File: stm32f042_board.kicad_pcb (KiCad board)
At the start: 4 copper layers, 37.8 x 18.8 mm, 25 parts, among them J1 Conn_01x12_Female, J2 Conn_01x12_Female, J3 USB_B_Micro, J5 JTAG/SWD, U1 STM32F042F6Px, U2 MCP1802, U3 USBLC6-2SC6

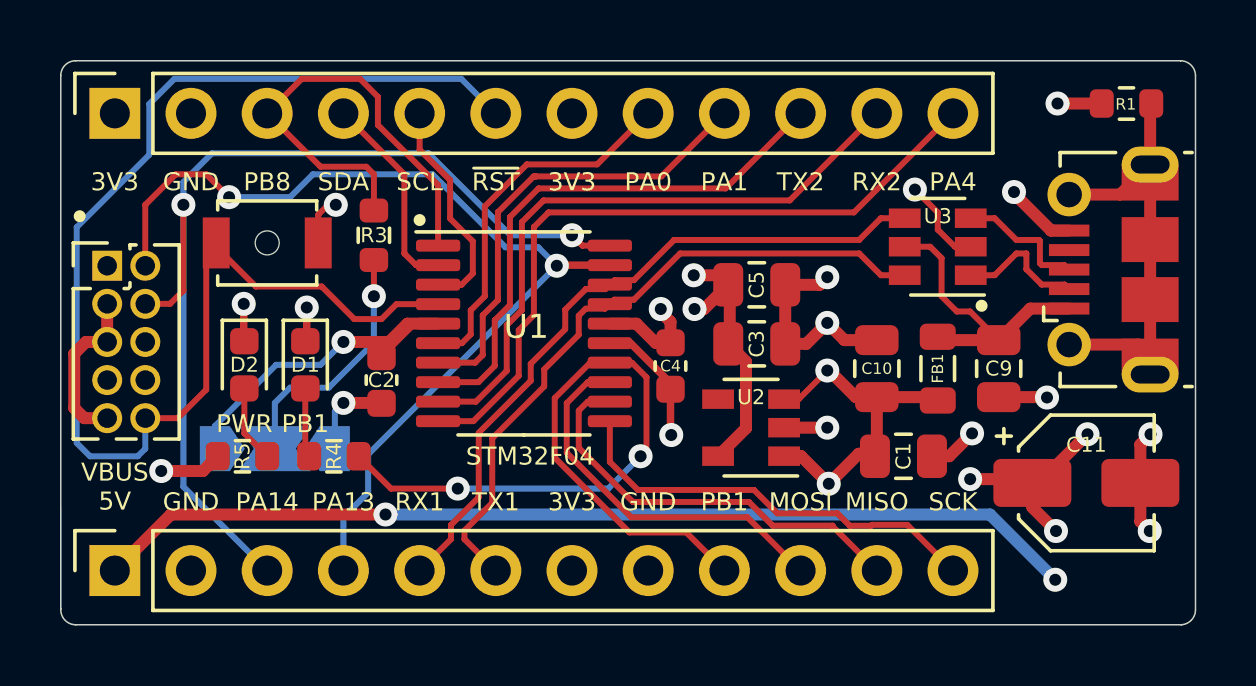
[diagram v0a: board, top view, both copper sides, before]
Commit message: Migrate to KiCad 7
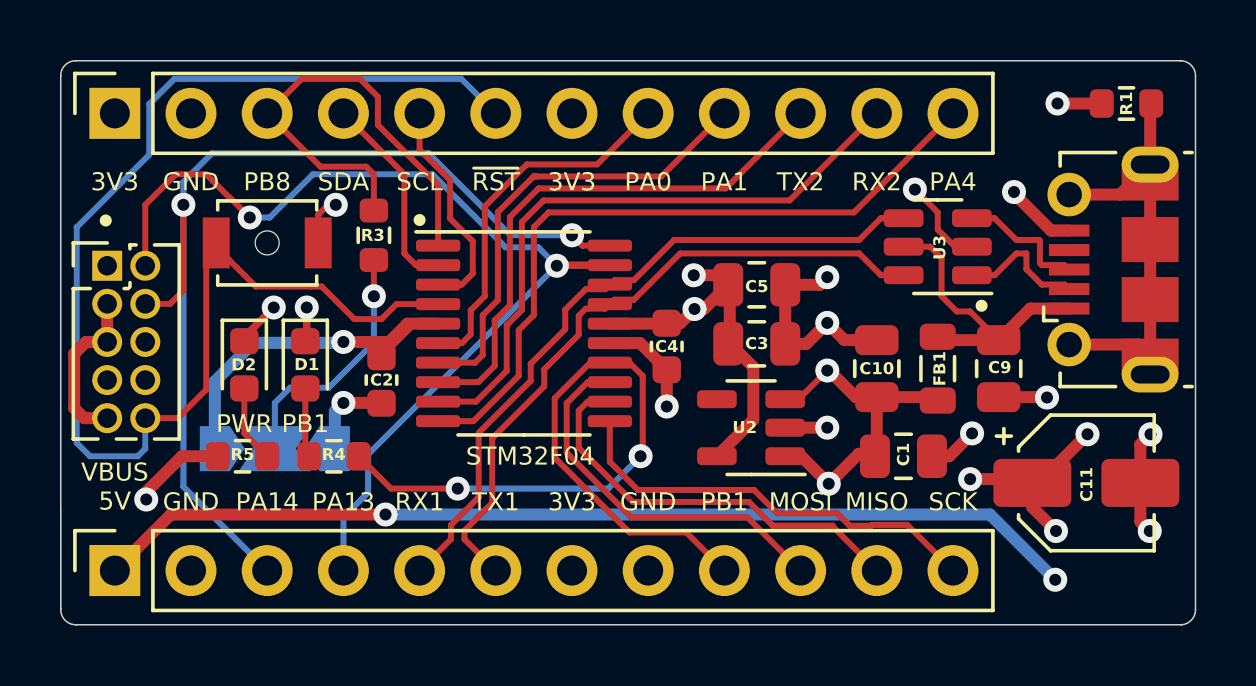
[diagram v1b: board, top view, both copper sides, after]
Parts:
- moved G*** 12.5 mm to (164.3, 68.6), turned to -90 degrees
- moved C4 0.66 mm to (161.4, 66.7)
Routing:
- net +3V3: track 26.2 -> 27.8 mm, vias 5 -> 4
- net SWDIO: track 32.9 -> 33.5 mm
- net GND: track 38.9 -> 38.4 mm

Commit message: Revert "Migrate to KiCad 7"
This reverts commit a80925b01a00ac2b6e233b577ff1a59522959ffa.

- Footprints and some other things don't seem to work right yet
- OSHPark not v7 compatible yet.
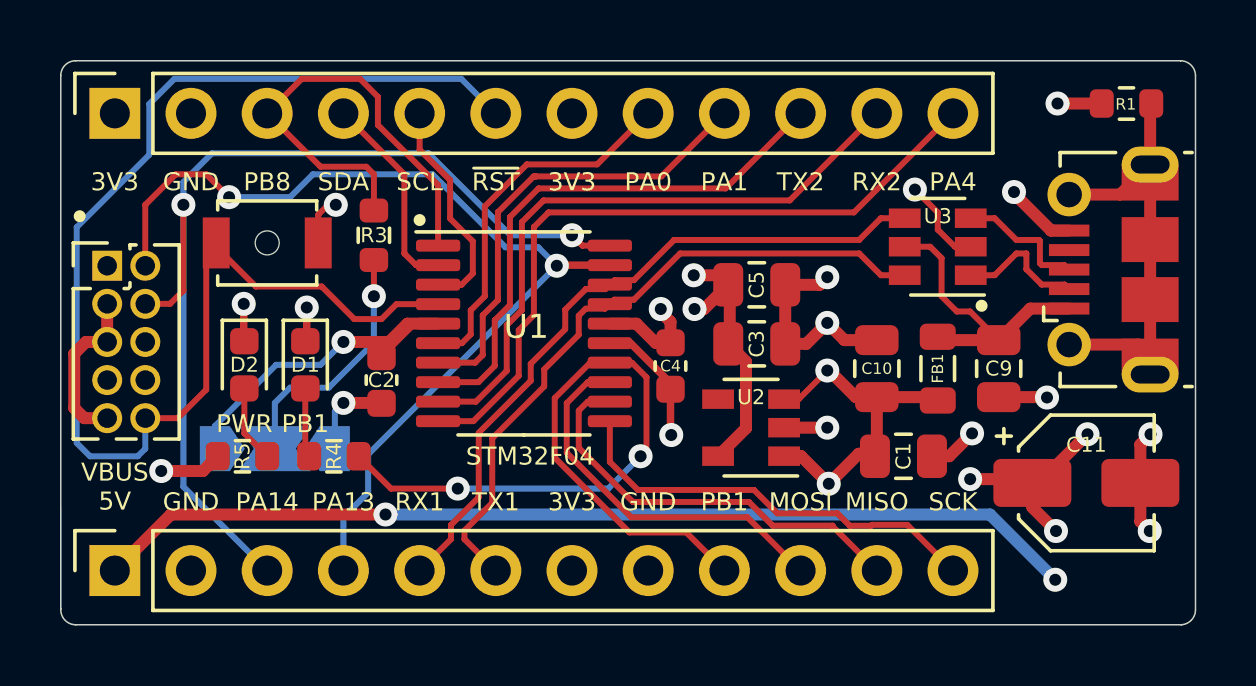
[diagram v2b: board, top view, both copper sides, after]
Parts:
- moved G*** 12.5 mm to (176.6, 70.4), turned to 0 degrees
- moved C4 0.66 mm to (161.5, 67.3)
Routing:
- net +3V3: track 27.8 -> 26.2 mm, vias 4 -> 5
- net SWDIO: track 33.5 -> 32.9 mm
- net GND: track 38.4 -> 38.9 mm
